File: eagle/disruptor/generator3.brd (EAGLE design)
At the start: 126.5 x 120.7 mm, 35 parts, among them IC1 NE555, IC2 74ALS04N, IC3 IR2110, IC4 7805TV, J1 PIN2F061.100, J2 PIN2F061.100, J3 PIN2F061.100, J4 PIN2F061.100, J5 PIN2F061.100, J6 PIN2F061.100, Q1 STP11NM60, Q2 STP11NM60

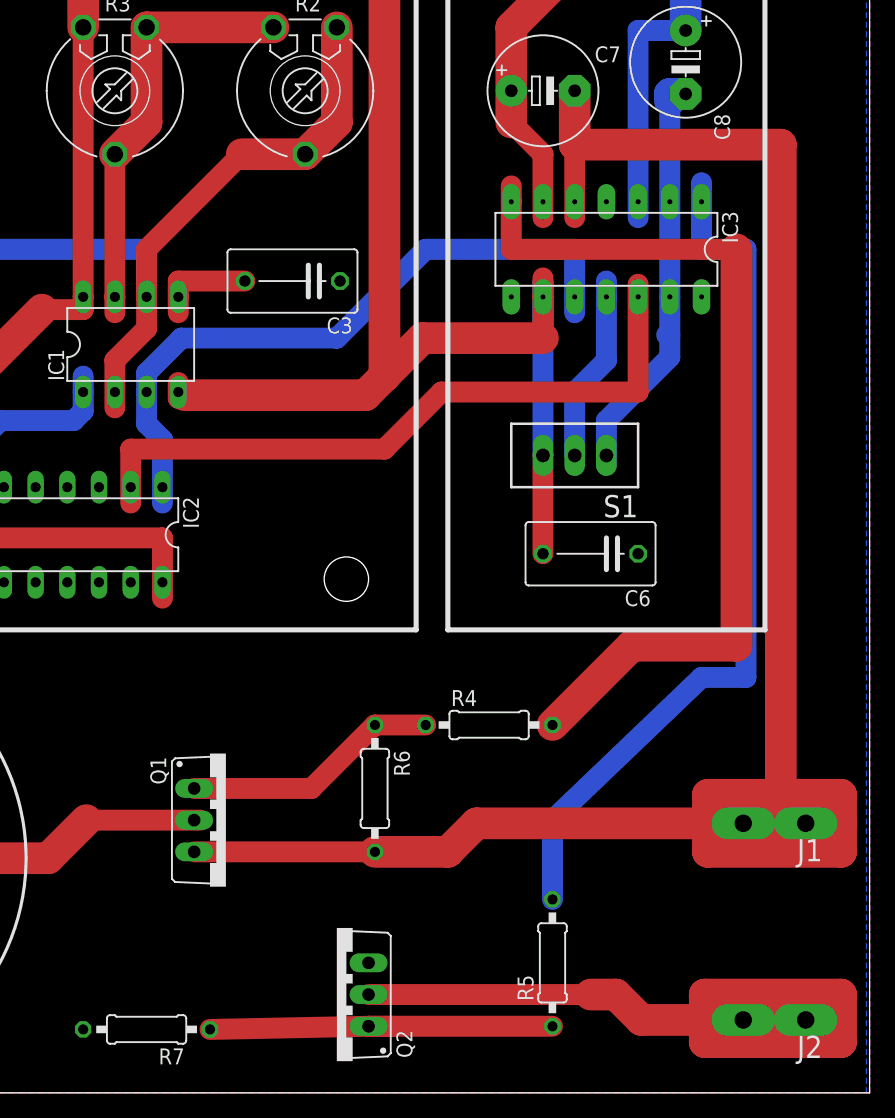
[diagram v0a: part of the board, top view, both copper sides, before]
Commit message: gen3
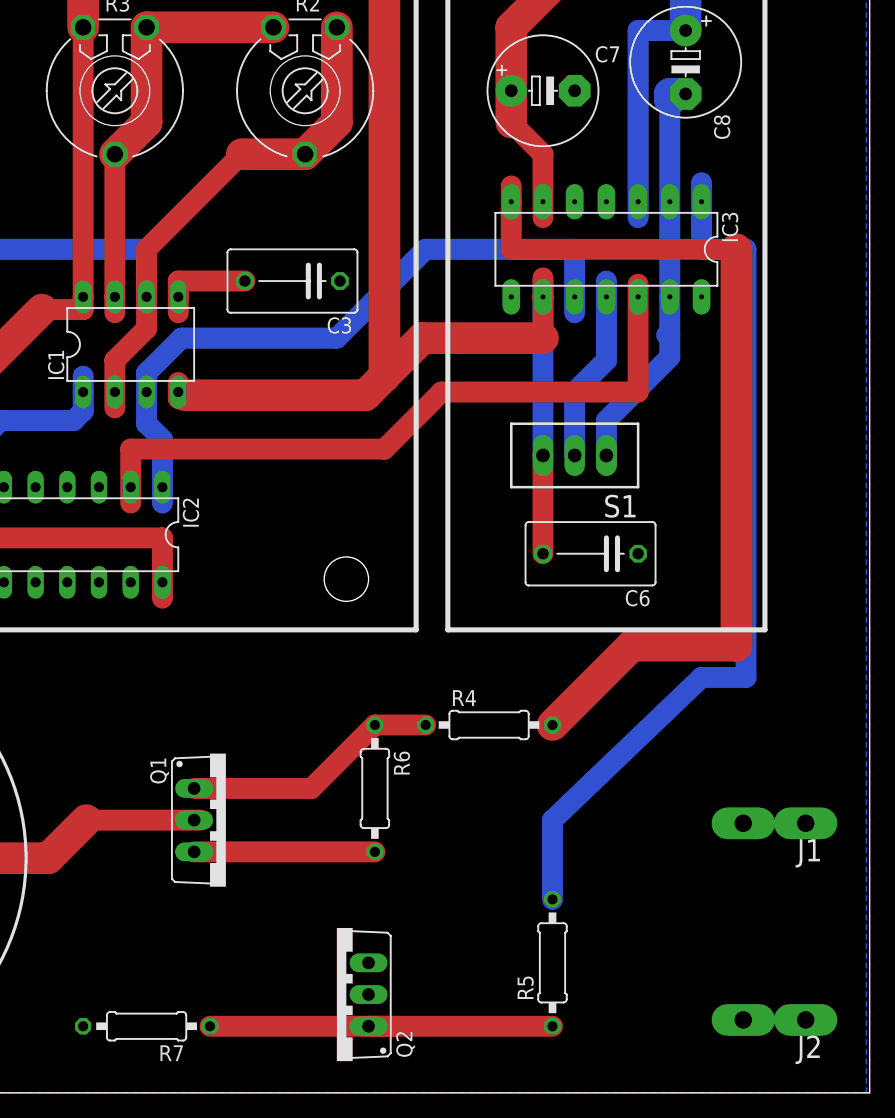
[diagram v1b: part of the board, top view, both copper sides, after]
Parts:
- moved R7 0.25 mm to (18.3, 5.08)
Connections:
- removed net TRANS1: C7.-, IC3.5, J1.A1, J1.A2, Q1.S, R6.2
- net GND: now also J2.A1, J2.A2
- net TRANS2: now also C7.-, IC3.5, J1.A1, J1.A2, Q1.S, R6.2; no longer J2.A1, J2.A2
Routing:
- net TRANS1: track 168.1 -> 0.00 mm
- net TRANS2: track 69.8 -> 14.5 mm
